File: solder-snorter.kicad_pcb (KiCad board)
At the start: 2 copper layers, 80 x 33.5 mm, 17 parts, among them J1 USB_B_Micro, M1 Fan, SW1 SW_SPDT, U1 MCP73831, U2 TLV61046A

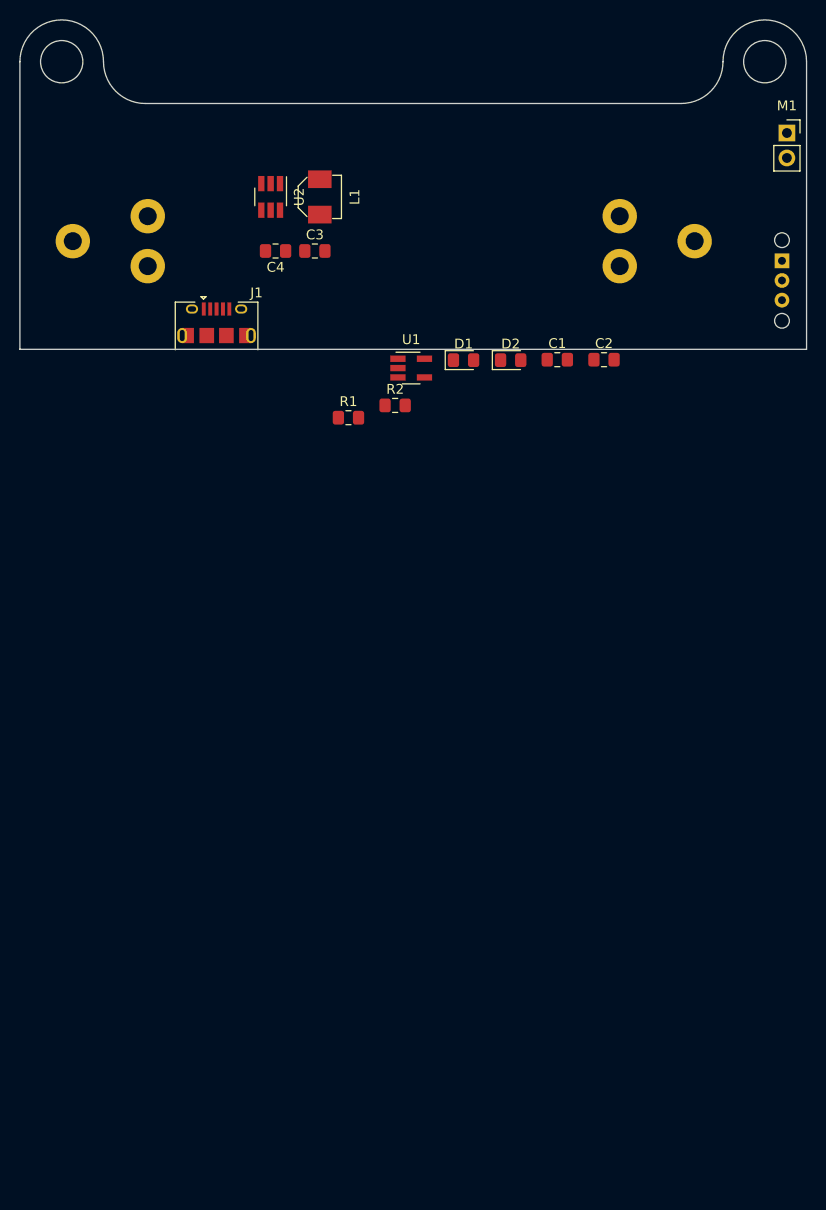
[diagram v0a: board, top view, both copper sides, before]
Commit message: Finished first cut at layout
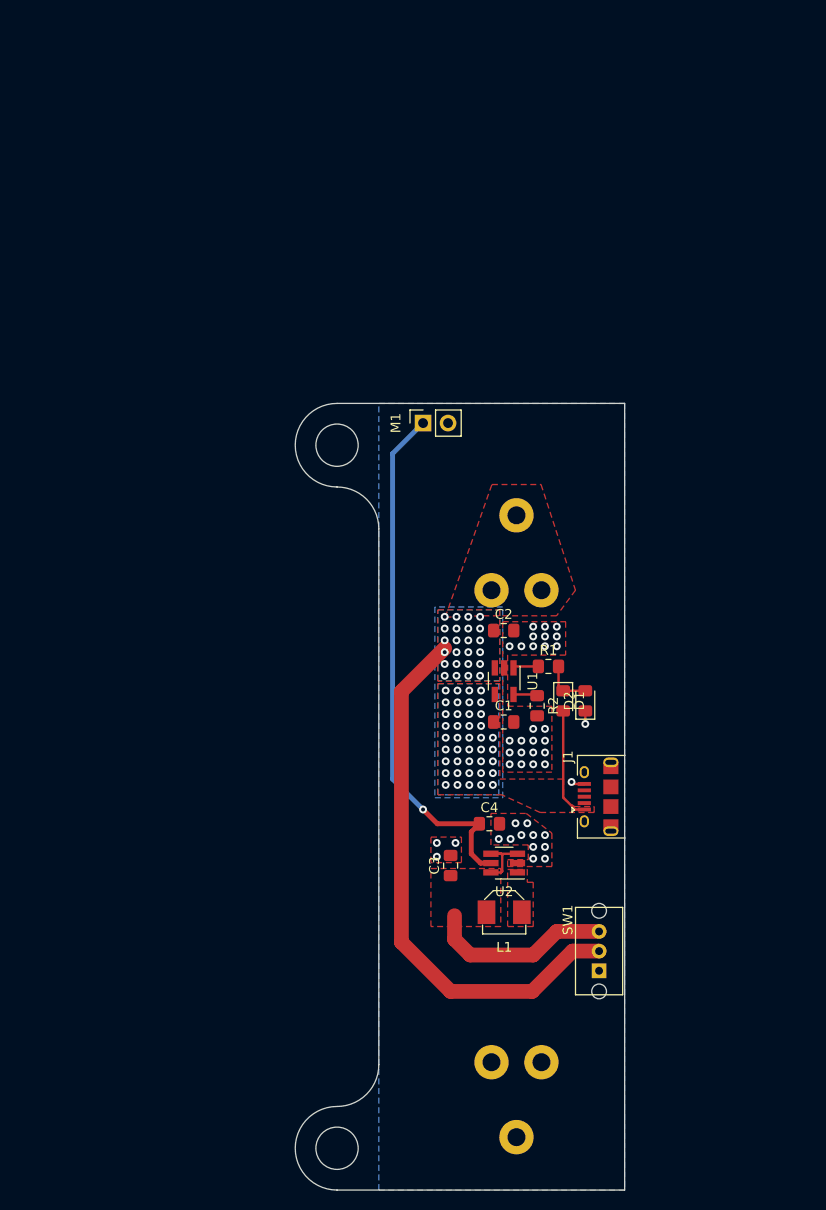
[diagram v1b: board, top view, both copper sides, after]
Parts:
- SW1: moved to F.Cu
- moved REF** 114.0 mm to (137.2, 151.2), turned to 90 degrees
- moved L1 75.1 mm to (154.2, 127.2), turned to 0 degrees
- moved U2 71.8 mm to (154.2, 122.2), turned to 180 degrees
- moved SW1 70.7 mm to (163.9, 131.2), turned to 90 degrees
- moved C3 64.0 mm to (148.8, 122.5), turned to 90 degrees
- moved C4 62.2 mm to (152.8, 118.2), turned to 0 degrees
- moved J1 62.1 mm to (162.4, 115.5), turned to 90 degrees
- moved BT1 61.0 mm to (155.5, 118.5), turned to 270 degrees
- moved REF** 58.4 mm to (137.2, 79.8), turned to 90 degrees
- moved M1 47.3 mm to (146.0, 77.5), turned to 90 degrees
- moved C1 37.2 mm to (154.2, 107.9)
- moved D1 36.1 mm to (160.2, 105.8), turned to 270 degrees
- moved D2 35.5 mm to (162.5, 105.8), turned to 90 degrees
- moved R2 33.8 mm to (157.6, 106.2), turned to 270 degrees
- moved U1 33.2 mm to (154.2, 103.8), turned to 270 degrees
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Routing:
- net VBAT: track 0.00 -> 55.6 mm, vias 0 -> 24
- net +12V: track 0.00 -> 54.0 mm, vias 0 -> 1
- net VBATSW: track 0.00 -> 25.5 mm
- net Net-(C1-Pad1): track 0.00 -> 11.5 mm, vias 0 -> 41
- net Net-(D1-Pad1): track 0.00 -> 4.92 mm
- net GND: track 0.00 -> 2.71 mm, vias 0 -> 41
- net Net-(R2-Pad1): track 0.00 -> 2.63 mm
- net Net-(R1-Pad1): track 0.00 -> 2.59 mm
- added copper zone on B.Cu, net GND
- added copper zone on F.Cu, net GND
- added copper zone on B.Cu, net Net-(C1-Pad1)
- added copper zone on F.Cu, net Net-(C1-Pad1)
- added copper zone on F.Cu, net Net-(L1-Pad2)
- added copper zone on B.Cu, net VBAT
- added copper zone on F.Cu, net VBAT
- added copper zone on F.Cu, net VBATSW
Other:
- board size 80 x 33.5 mm -> 33.5 x 80 mm
- net class Default: clearance 0.2 -> 0.25
- net class Min added: clearance 0.1, trace_width 0.1, via_dia 0.45, via_drill 0.2
- rule pad_to_mask_clearance: 0.05 -> 0
- rule trace_clearance: 0.2 -> 0.25
- rule trace_min: 0.2 -> 0.1
- rule via_min_drill: 0.3 -> 0.2
- rule via_min_size: 0.4 -> 0.45
